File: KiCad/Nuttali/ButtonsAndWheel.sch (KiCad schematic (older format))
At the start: 23 parts, among them J3 Conn_01x03_Male, J4 Conn_01x02_Male, SW8 Rotary_Encoder, U6 Button, U7 Button, U8 Scroll_button, U9 Button

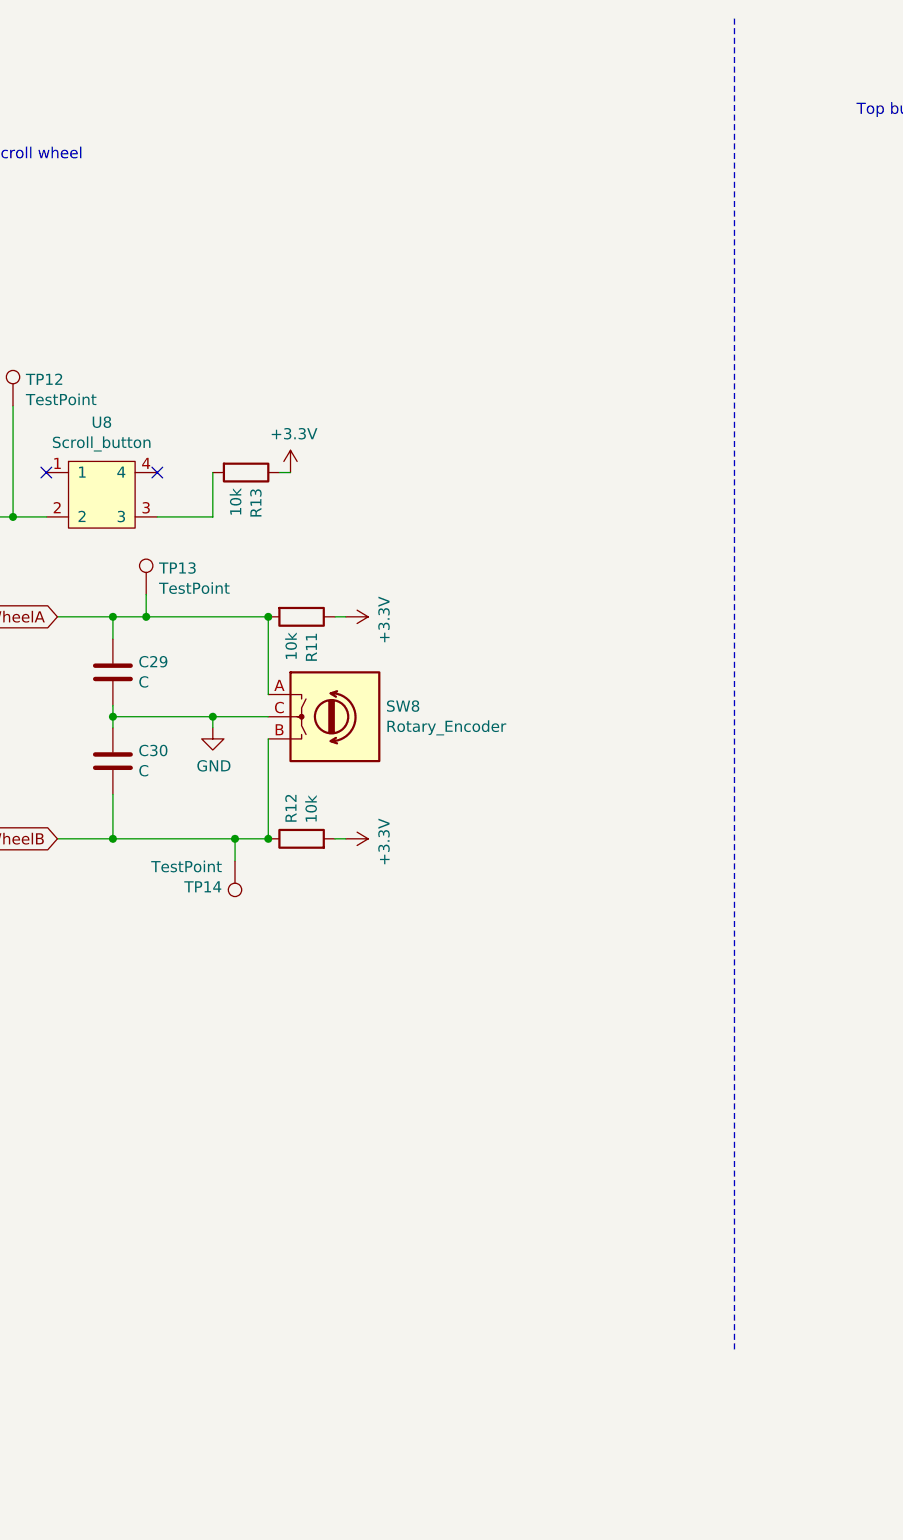
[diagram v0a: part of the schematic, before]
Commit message: Last push befor ordering
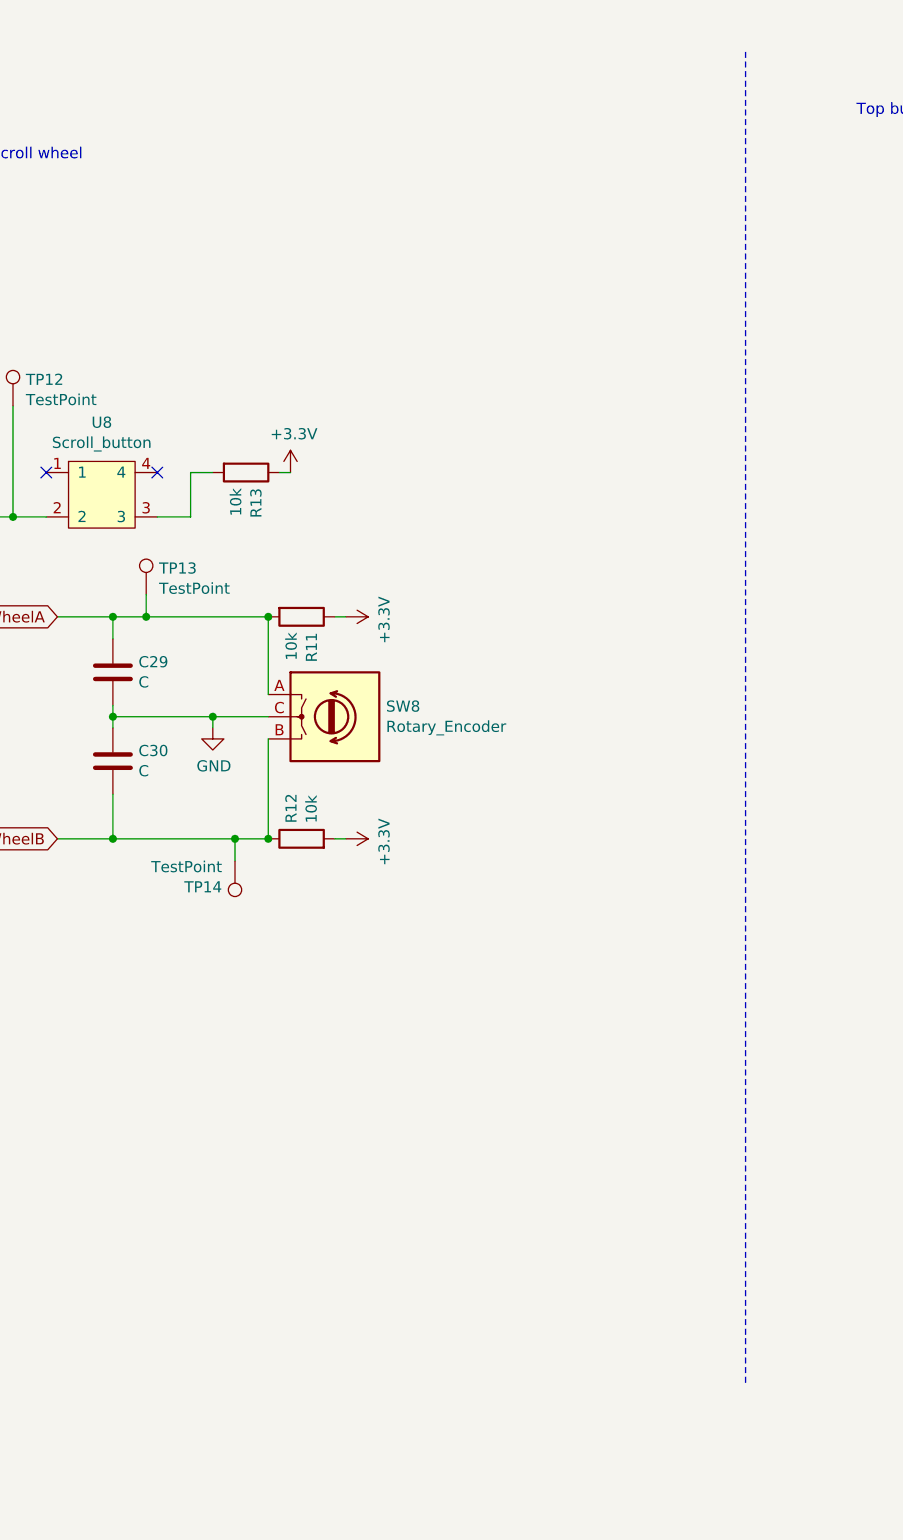
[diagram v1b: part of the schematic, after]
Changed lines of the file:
@@
 	1    0    0    -1
 $EndComp
+NoConn ~ 4400 2550
 NoConn ~ 3900 2550
 $Comp
@@
 NoConn ~ 9500 3400
 Wire Notes Line
-	7000 6500 7000 500
+	7050 6650 7050 650
 Wire Wire Line
 	9350 3400 9350 3700
@@
 	4750 4200 4900 4200
 Wire Wire Line
-	4650 2750 4400 2750
-Wire Wire Line
-	4650 2750 4650 2550
-NoConn ~ 4400 2550
+	4400 2750 4550 2750
+Wire Wire Line
+	4550 2750 4550 2550
+Wire Wire Line
+	4550 2550 4650 2550
 $EndSCHEMATC

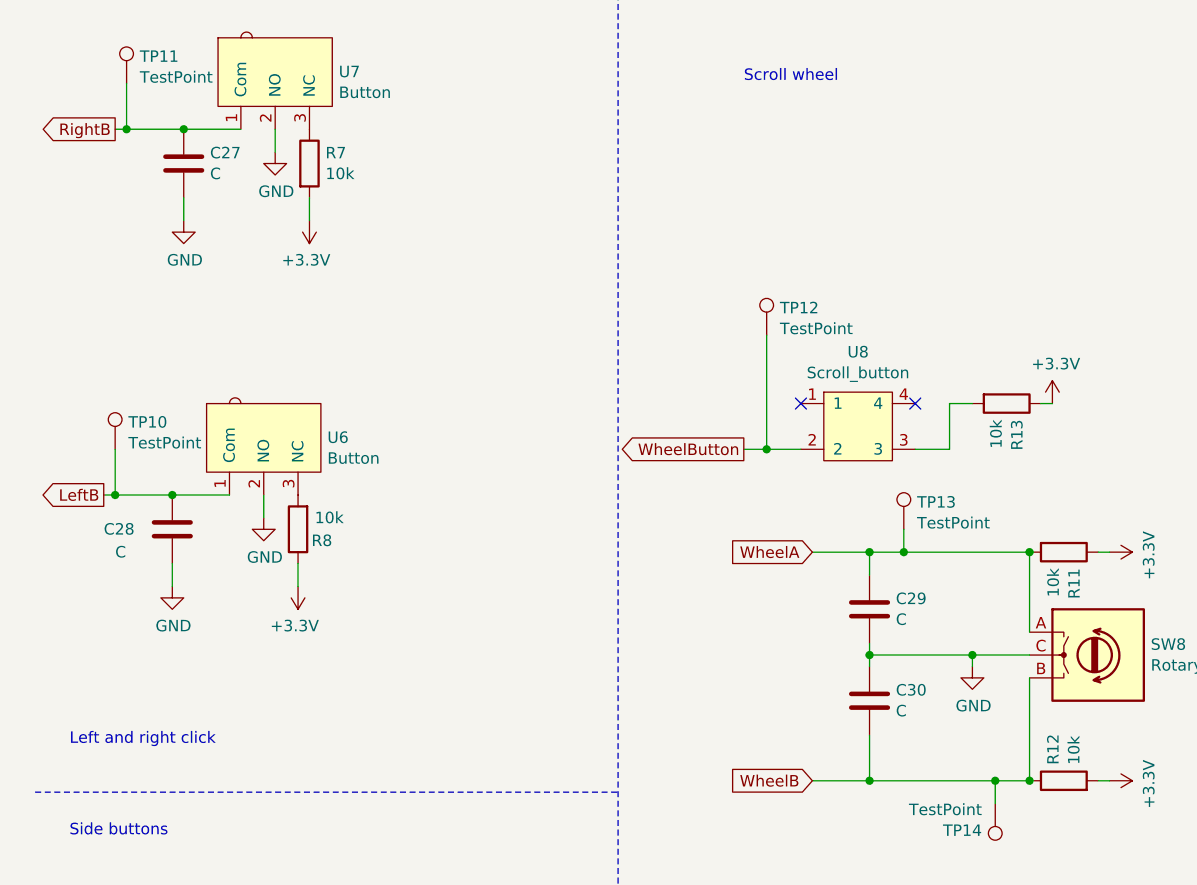
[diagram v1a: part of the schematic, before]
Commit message: added pers things to project
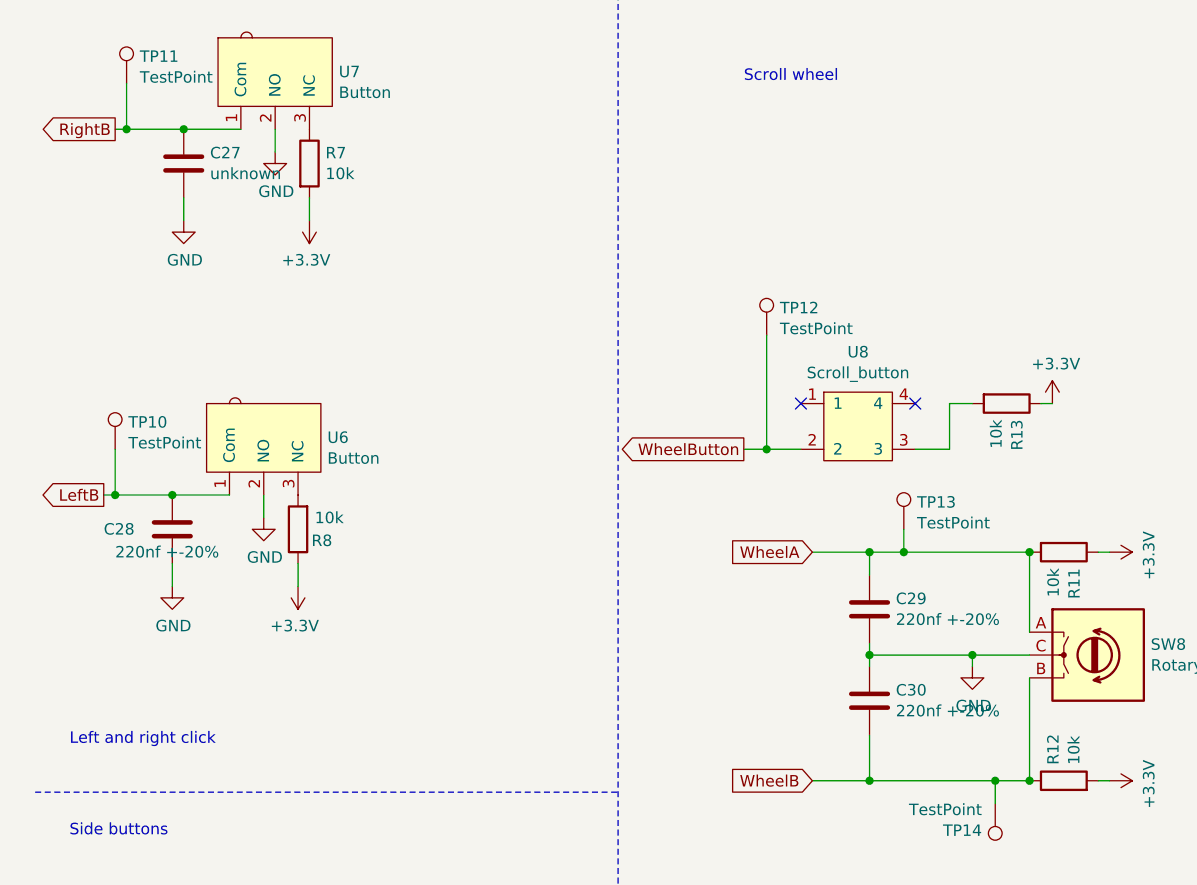
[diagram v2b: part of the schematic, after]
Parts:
- C27: value C -> unknown
- C28, C29, C30: value C -> 220nf +-20%
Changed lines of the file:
@@
 P 1150 3100
 F 0 "C28" H 850 3100 50  0000 L CNN
-F 1 "C" H 900 3000 50  0000 L CNN
+F 1 "220nf +-20%" H 900 3000 50  0000 L CNN
 F 2 "Capacitor_SMD:C_0805_2012Metric_Pad1.18x1.45mm_HandSolder" H 1188 2950 50  0001 C CNN
 F 3 "~" H 1150 3100 50  0001 C CNN
@@
 P 4200 3450
 F 0 "C29" H 4315 3496 50  0000 L CNN
-F 1 "C" H 4315 3405 50  0000 L CNN
+F 1 "220nf +-20%" H 4315 3405 50  0000 L CNN
 F 2 "Capacitor_SMD:C_0805_2012Metric_Pad1.18x1.45mm_HandSolder" H 4238 3300 50  0001 C CNN
 F 3 "~" H 4200 3450 50  0001 C CNN
@@
 P 4200 3850
 F 0 "C30" H 4315 3896 50  0000 L CNN
-F 1 "C" H 4315 3805 50  0000 L CNN
+F 1 "220nf +-20%" H 4315 3805 50  0000 L CNN
 F 2 "Capacitor_SMD:C_0805_2012Metric_Pad1.18x1.45mm_HandSolder" H 4238 3700 50  0001 C CNN
 F 3 "~" H 4200 3850 50  0001 C CNN
@@
 P 1200 1500
 F 0 "C27" H 1315 1546 50  0000 L CNN
-F 1 "C" H 1315 1455 50  0000 L CNN
+F 1 "unknown" H 1315 1455 50  0000 L CNN
 F 2 "Capacitor_SMD:C_0805_2012Metric_Pad1.18x1.45mm_HandSolder" H 1238 1350 50  0001 C CNN
 F 3 "~" H 1200 1500 50  0001 C CNN
